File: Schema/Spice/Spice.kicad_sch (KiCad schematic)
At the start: 5 parts, among them J1 Conn_02x03_Top_Bottom, U1 ATtiny85V-10P

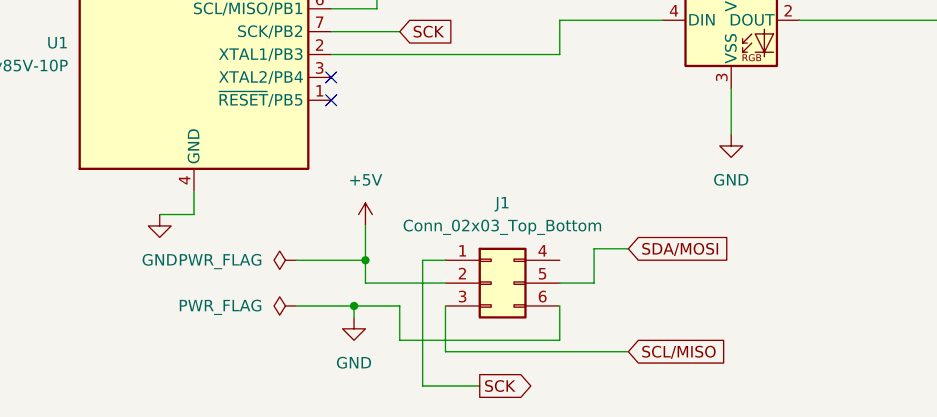
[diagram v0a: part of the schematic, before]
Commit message: Räume Schema auf
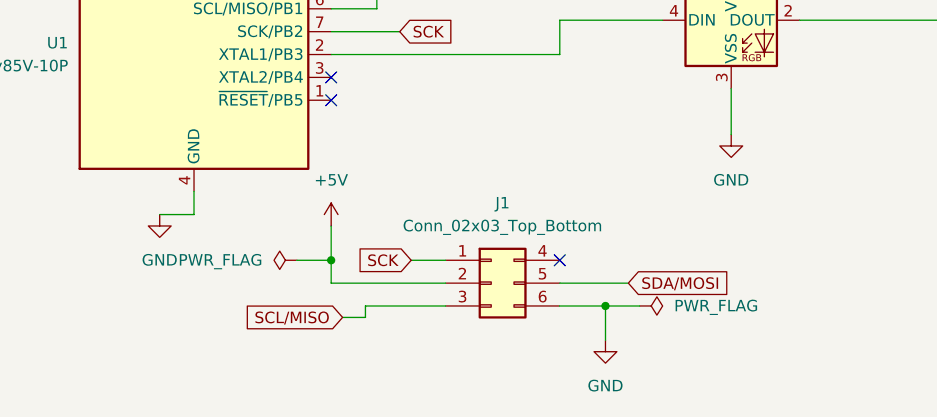
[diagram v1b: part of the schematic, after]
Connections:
- no-connect marks 3 -> 4
